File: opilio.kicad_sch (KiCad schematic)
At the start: 87 parts, among them J1 Screw_Terminal_01x02, J2 USB_B_Micro, J3 Conn_01x02_Male, J4 Conn_01x02_Male, J5 Conn_01x02_Male, Q1 PMV25ENEAR, Q2 AO3401A, U1 EUP3458, U2 STM32F103C8T6, Y1 YSX531SL 8MHz, Y2 YST310S 32.768KHz

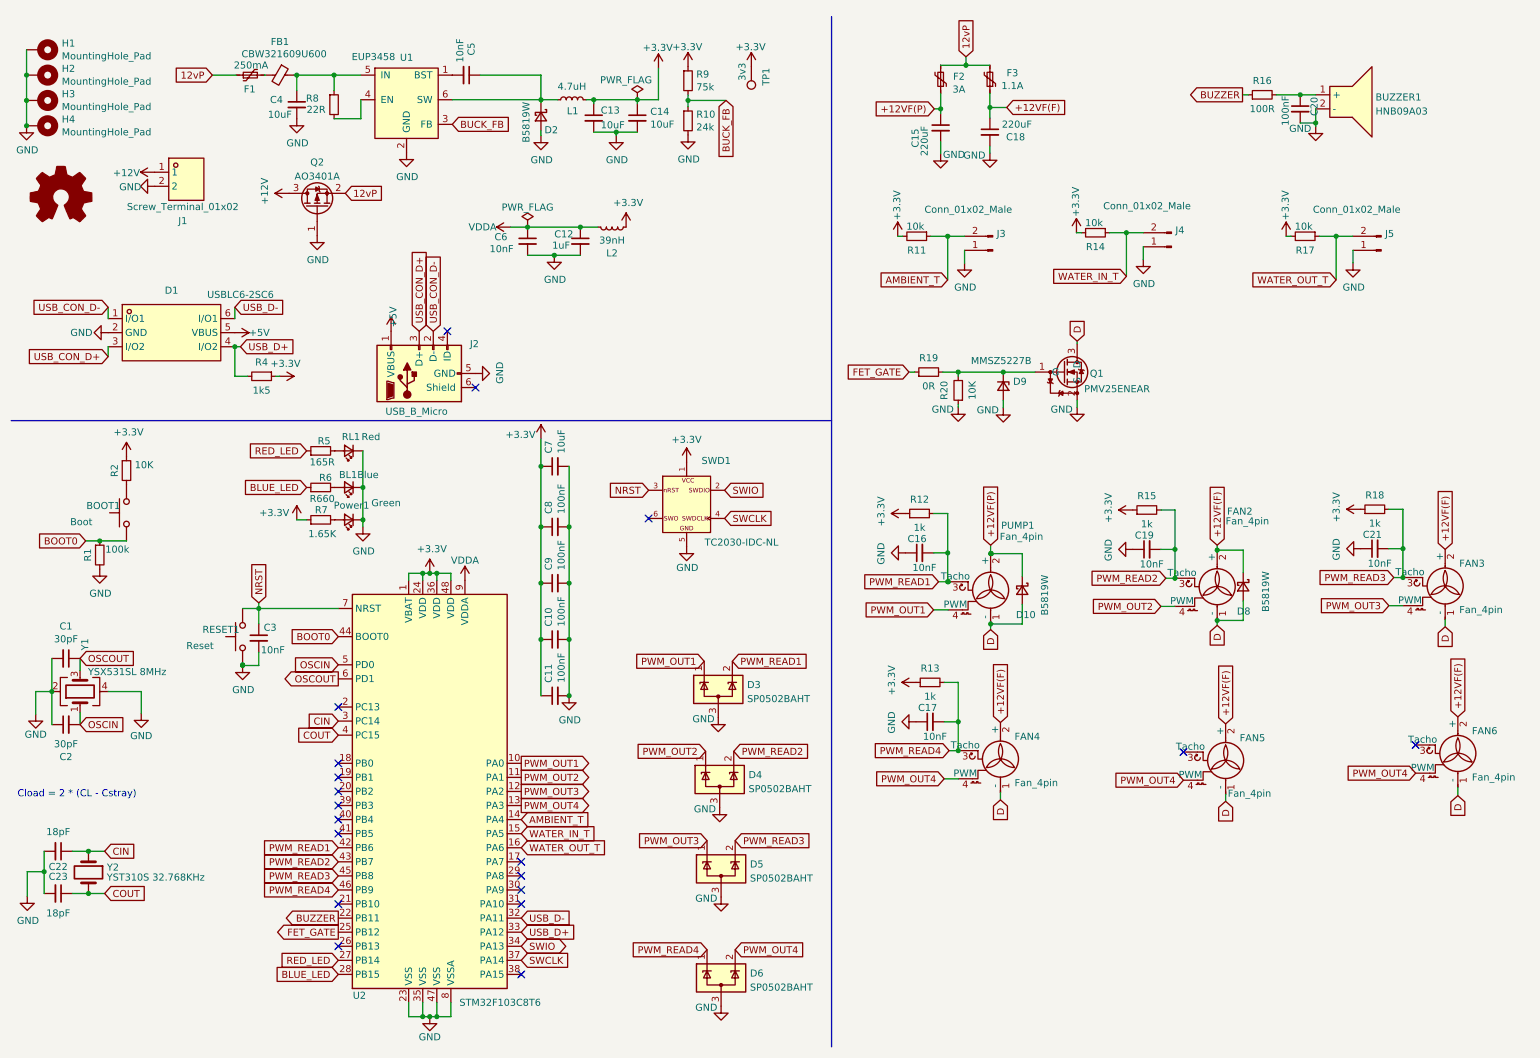
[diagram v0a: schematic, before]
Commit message: cleanup and annotate schema
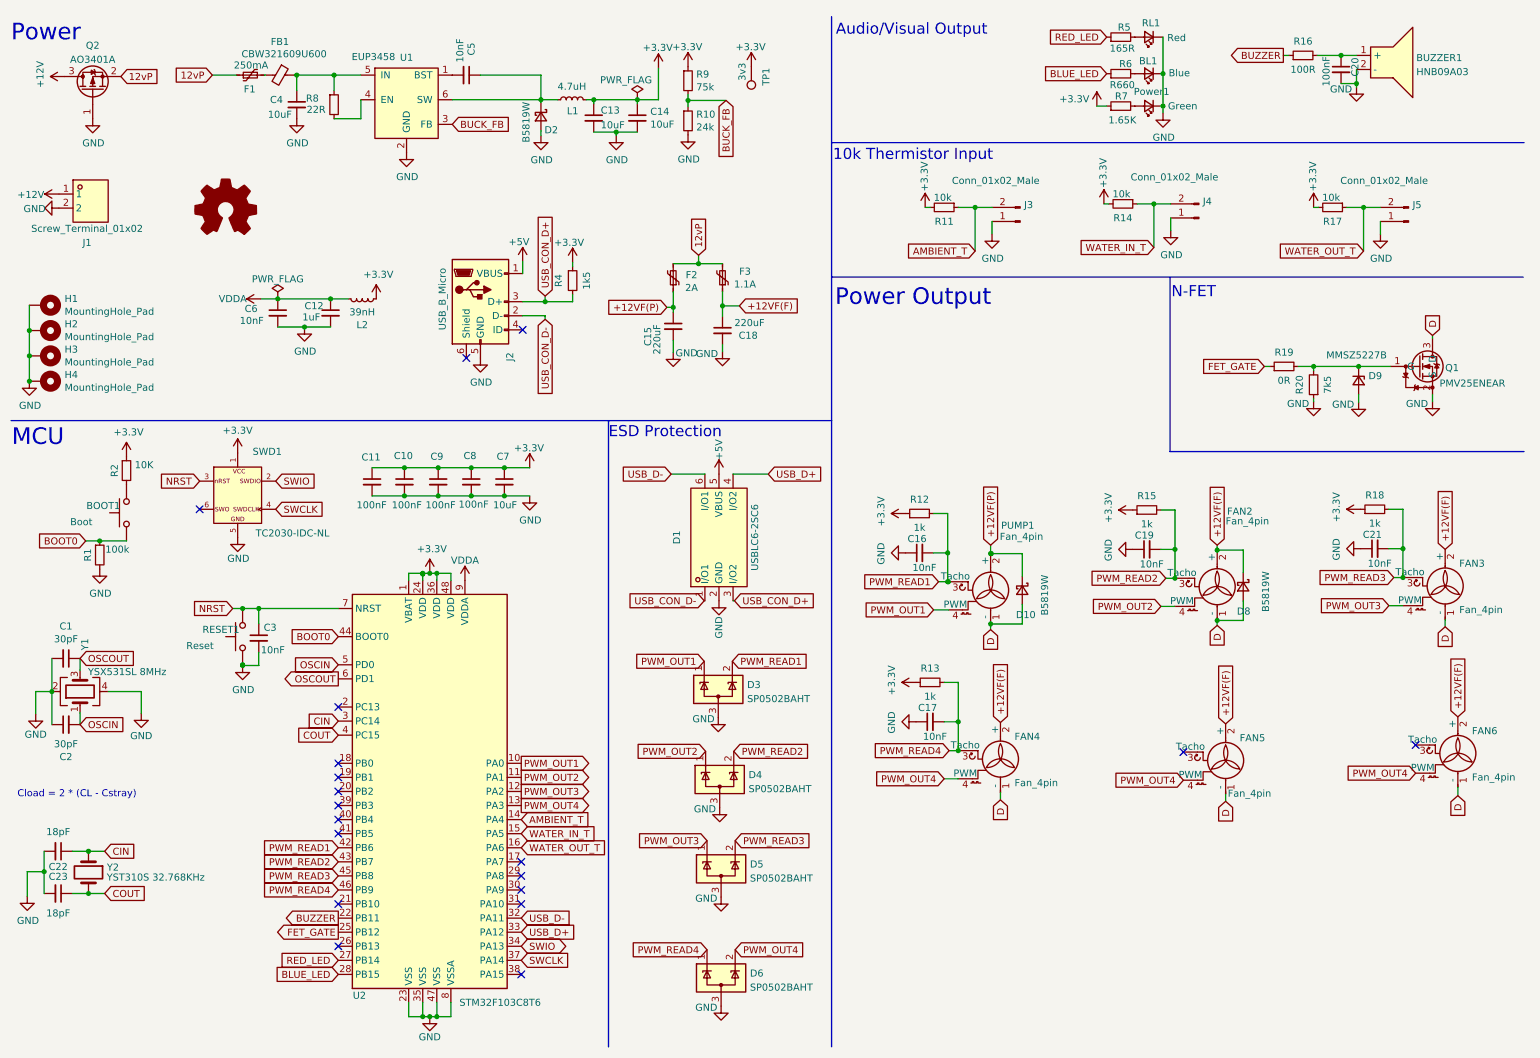
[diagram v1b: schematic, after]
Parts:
- F2: value 3A -> 2A; footprint Fuse:Fuse_1812_4532Metric_Pad1.30x3.40mm_HandSolder -> Fuse:Fuse_1206_3216Metric_Pad1.42x1.75mm_HandSolder
- R20: value 10K -> 7k5
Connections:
- net USB_CON_D+: now also R4.2
- net USB_D+: no longer R4.2
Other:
- note added: "10k Thermistor Input"
- note added: "Audio/Visual Output"
- note added: "ESD Protection"
- note added: "MCU"
- note added: "N-FET"
- note added: "Power"
- note added: "Power Output"
- moved on the sheet: BL1, BUZZER1, C10, C11, C12, C15, C18, C20, C6, C7, C8, C9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

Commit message: WIP:0402
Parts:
- C1, C10, C11, C16, C17, C19, C2, C20, C21, C22, C23, C3, C6, C8, C9: footprint Capacitor_SMD:C_0603_1608Metric_Pad1.08x0.95mm_HandSolder -> Capacitor_SMD:C_0402_1005Metric_Pad0.74x0.62mm_HandSolder
- R1, R10, R11, R12, R13, R14, R15, R16, R17, R18, R2, R20, R4, R5, R6, R7, R8, R9: footprint Resistor_SMD:R_0603_1608Metric_Pad0.98x0.95mm_HandSolder -> Resistor_SMD:R_0402_1005Metric_Pad0.72x0.64mm_HandSolder
